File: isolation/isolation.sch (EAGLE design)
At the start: 4 parts

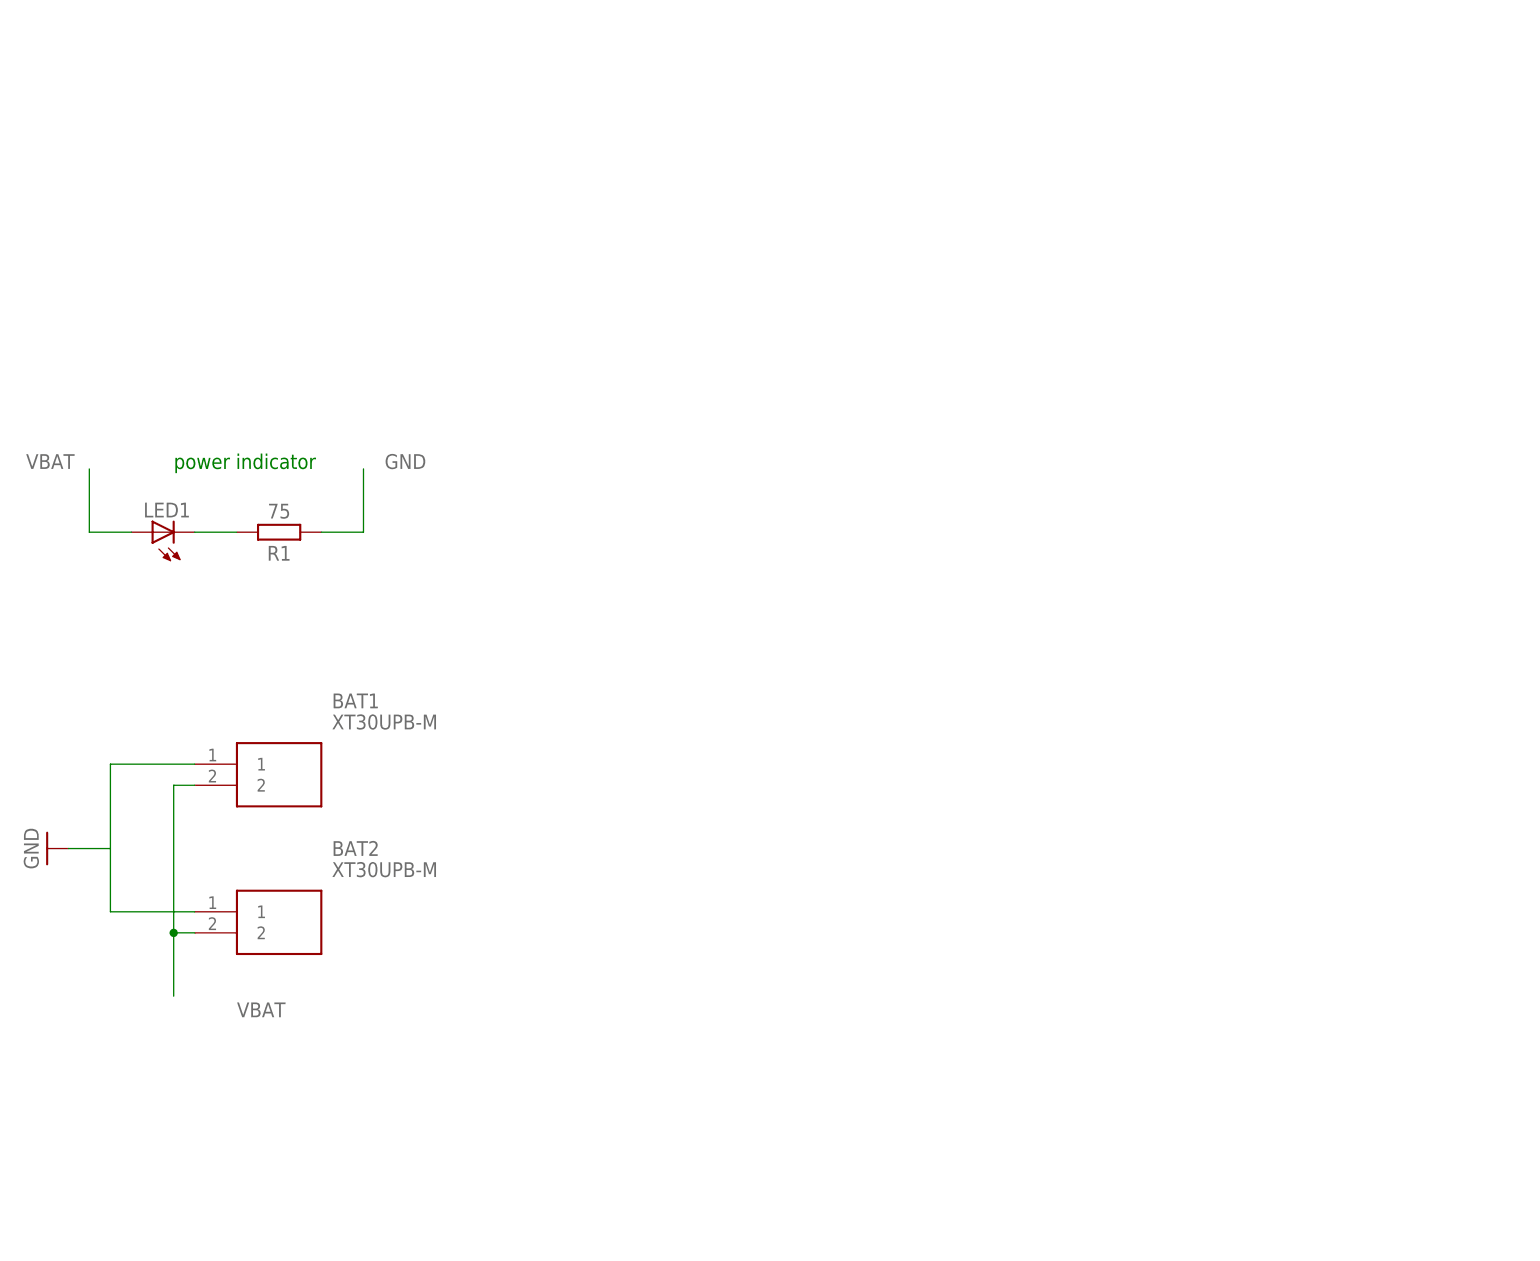
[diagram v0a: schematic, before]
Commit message: 12v boost schematic complete
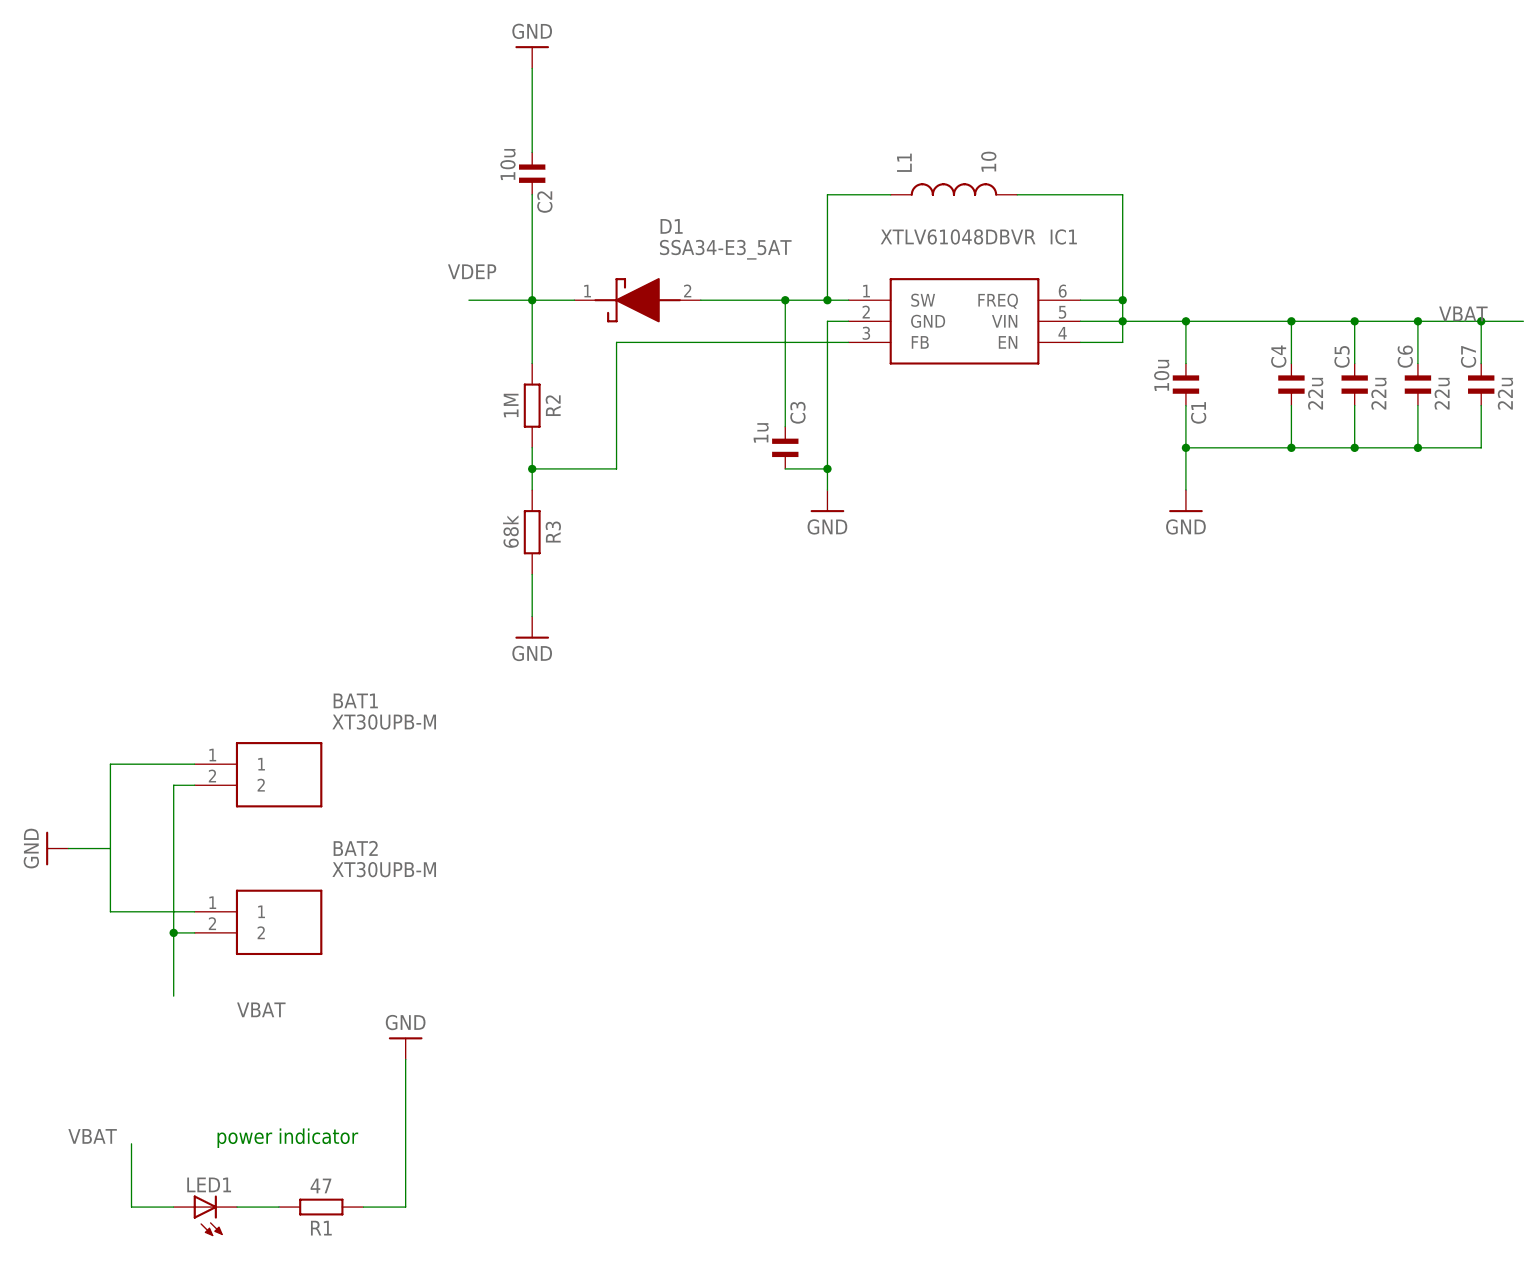
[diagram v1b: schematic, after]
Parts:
- added C1, C2: 10u, 52101-101-REV-A_v16:RC-MASTER-SMD_C_0603MP
- added C3: 1u, 52101-101-REV-A_v16:RC-MASTER-SMD_C_0603MP
- added C4, C5, C6, C7: 22u, 52101-101-REV-A_v16:RC-MASTER-SMD_C_0603MP
- added D1: SSA34-E3_5AT, SamacSys_Parts:SSA34-E3_5AT
- added IC1: XTLV61048DBVR, SamacSys_Parts:XTLV61048DBVR
- added L1: 10, BeagleBone_Blue_R3:INDUCTOR
- added R2: 1M, Resistor:R_CHIP-0603(1608-METRIC)
- added R3: 68k, Resistor:R_CHIP-0603(1608-METRIC)
- R1: value 75 -> 47
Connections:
- new net N$2: C3.1, D1.A, IC1.SW, L1.1
- new net N$3: IC1.FB, R2.2, R3.1
- new net VDEP: C2.2, D1.K, R2.1
- net GND: now also C1.2, C2.1, C3.2, C4.1, C5.1, C6.1, C7.1, IC1.GND, R3.2
- net VBAT: now also C1.1, C4.2, C5.2, C6.2, C7.2, IC1.EN, IC1.FREQ, IC1.VIN, L1.2
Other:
- moved on the sheet: LED1, R1
